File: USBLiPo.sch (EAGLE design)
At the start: 15 parts, among them IC1 LTC4054, Q1 2N7002, X1 USBSF-MICROB

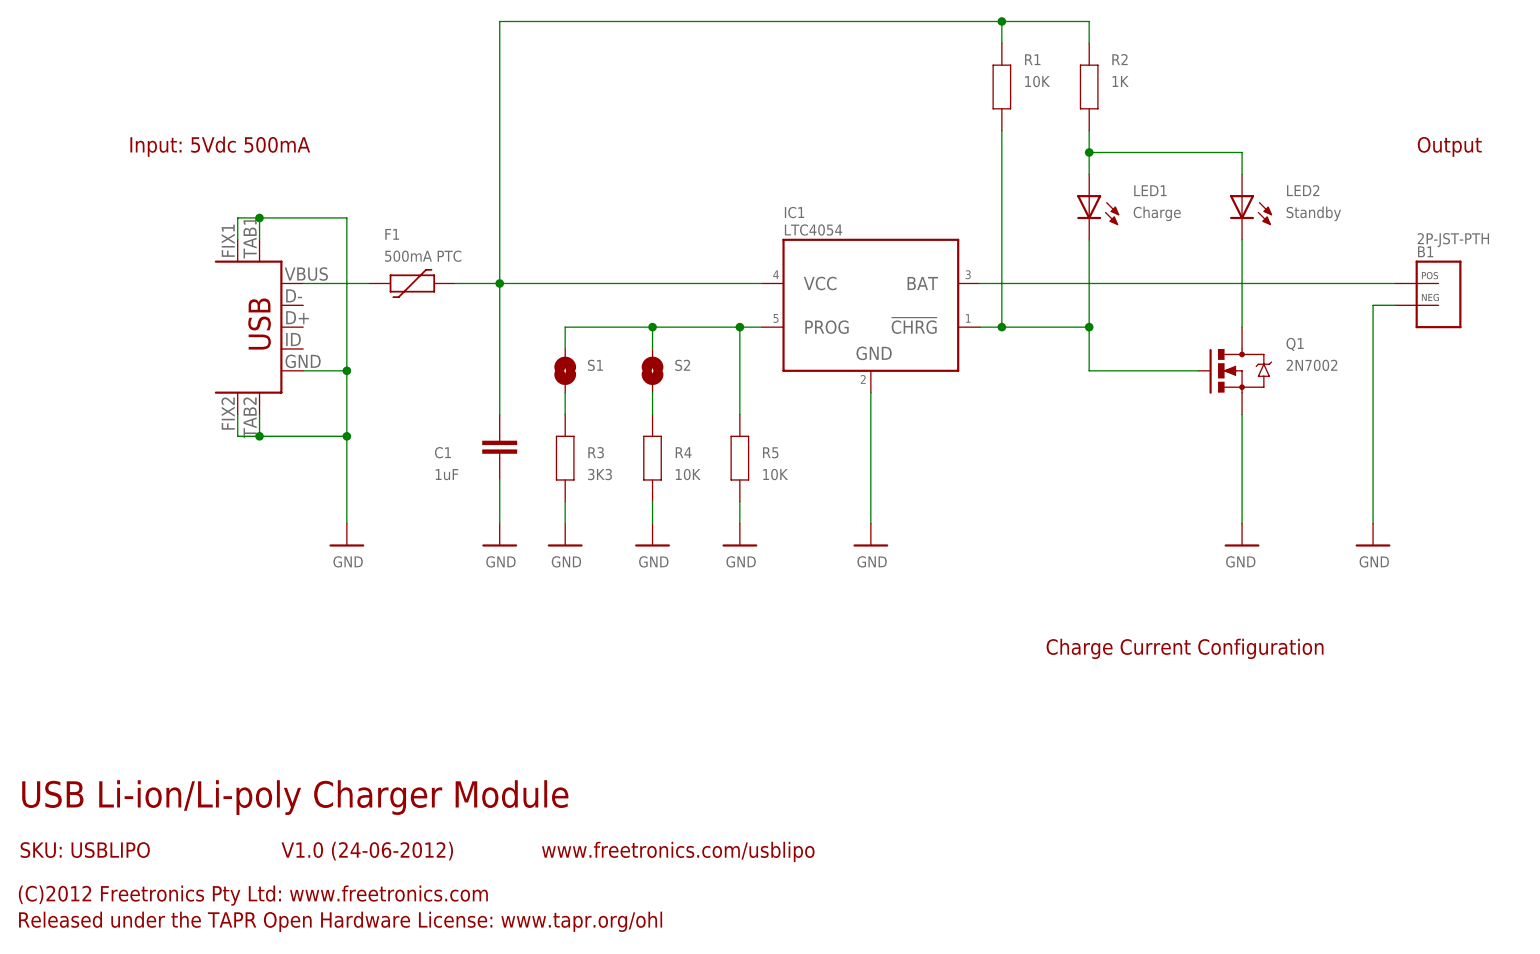
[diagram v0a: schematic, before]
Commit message: Final changes for v1.0 release
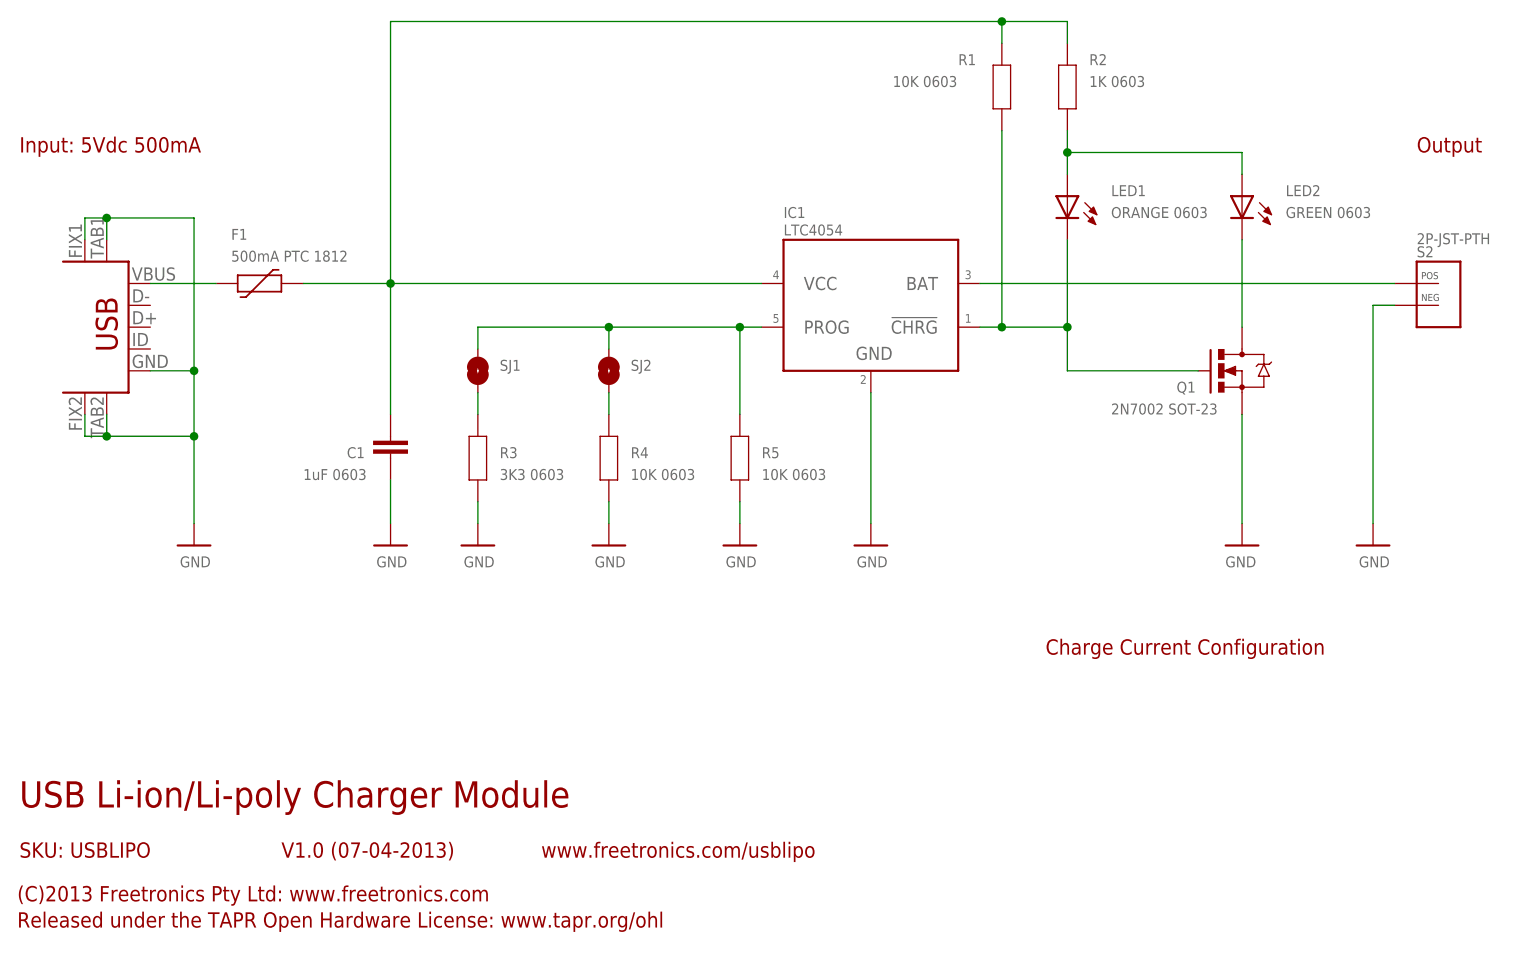
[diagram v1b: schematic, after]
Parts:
- removed B1: 2P-JST-PTH, freetronics-jon:FREETRONICS-LUKE_2P-JST-TH-RAPTH
- removed X1: USBSF-MICROB, freetronics-jon:USBSF-MICROB
- added SJ1, SJ2: SJ, freetronics-luke:SJ
- C1: value 1uF -> 1uF 0603
- F1: value 500mA PTC -> 500mA PTC 1812
- LED1: value Charge -> ORANGE 0603
- LED2: value Standby -> GREEN 0603
- Q1: value 2N7002 -> 2N7002 SOT-23
- R1, R4, R5: value 10K -> 10K 0603
- R2: value 1K -> 1K 0603
- R3: value 3K3 -> 3K3 0603
- S1: value SJ -> USBSF-MICROB; device freetronics-luke:SJ -> freetronics-jon:USBSF-MICROB
- S2: value SJ -> 2P-JST-PTH; device freetronics-luke:SJ -> freetronics-jon:FREETRONICS-LUKE_2P-JST-TH-RAPTH
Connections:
- net GND: now also S1.FIX1, S1.FIX2, S1.GND, S1.TAB1, S1.TAB2, S2.NEG; no longer B1.NEG, X1.FIX1, X1.FIX2, X1.GND, X1.TAB1, X1.TAB2
- net N$113: now also S1.VBUS; no longer X1.VBUS
- net N$3: now also SJ1.2, SJ2.2; no longer S1.2, S2.2
- net N$4: now also S2.POS; no longer B1.POS
- net N$5: now also SJ1.1; no longer S1.1
- net N$7: now also SJ2.1; no longer S2.1
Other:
- note added: "(C)2013 Freetronics Pty Ltd: www.freetronics.com"
- note added: "Charge"
- note added: "SJ1"
- note added: "SJ2"
- note added: "Standby"
- note added: "V1.0 (07-04-2013)"
- note removed: "(C)2012 Freetronics Pty Ltd: www.freetronics.com"
- note removed: "0603"
- note removed: "1812"
- note removed: "Green"
- note removed: "S1"
- note removed: "S2"
- note removed: "SOT-23"
- note removed: "V1.0 (24-06-2012)"
- note removed: "Yellow"
- moved on the sheet: C1, F1, LED1, R2, R3, R4
